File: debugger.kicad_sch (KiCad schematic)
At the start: 29 parts, among them J5 SM03B-SRSS-TB, J7 Conn_ARM_JTAG_SWD_10, J8 Conn_ST_STDC14, J9 SM03B-SRSS-TB

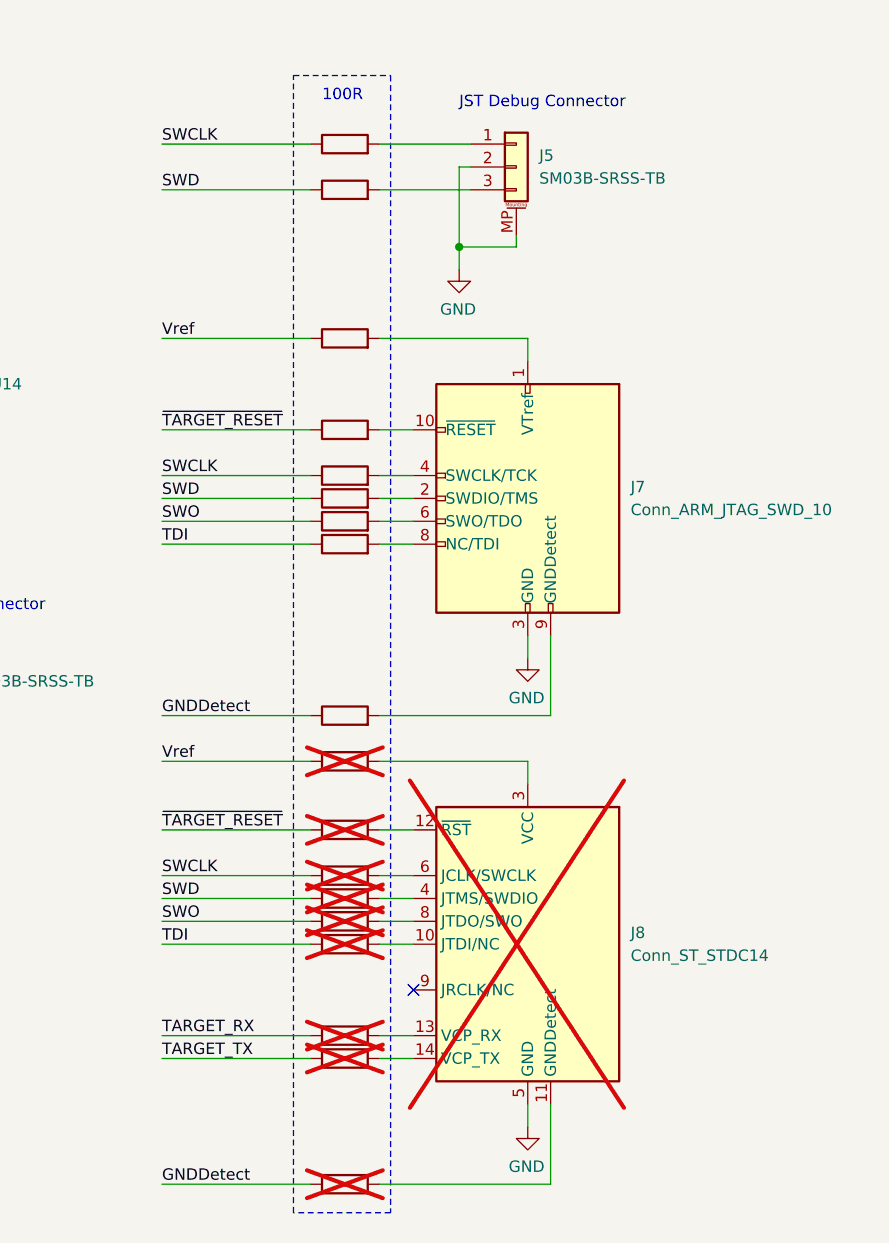
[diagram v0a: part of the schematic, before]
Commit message: Layout Tester and USB Hub
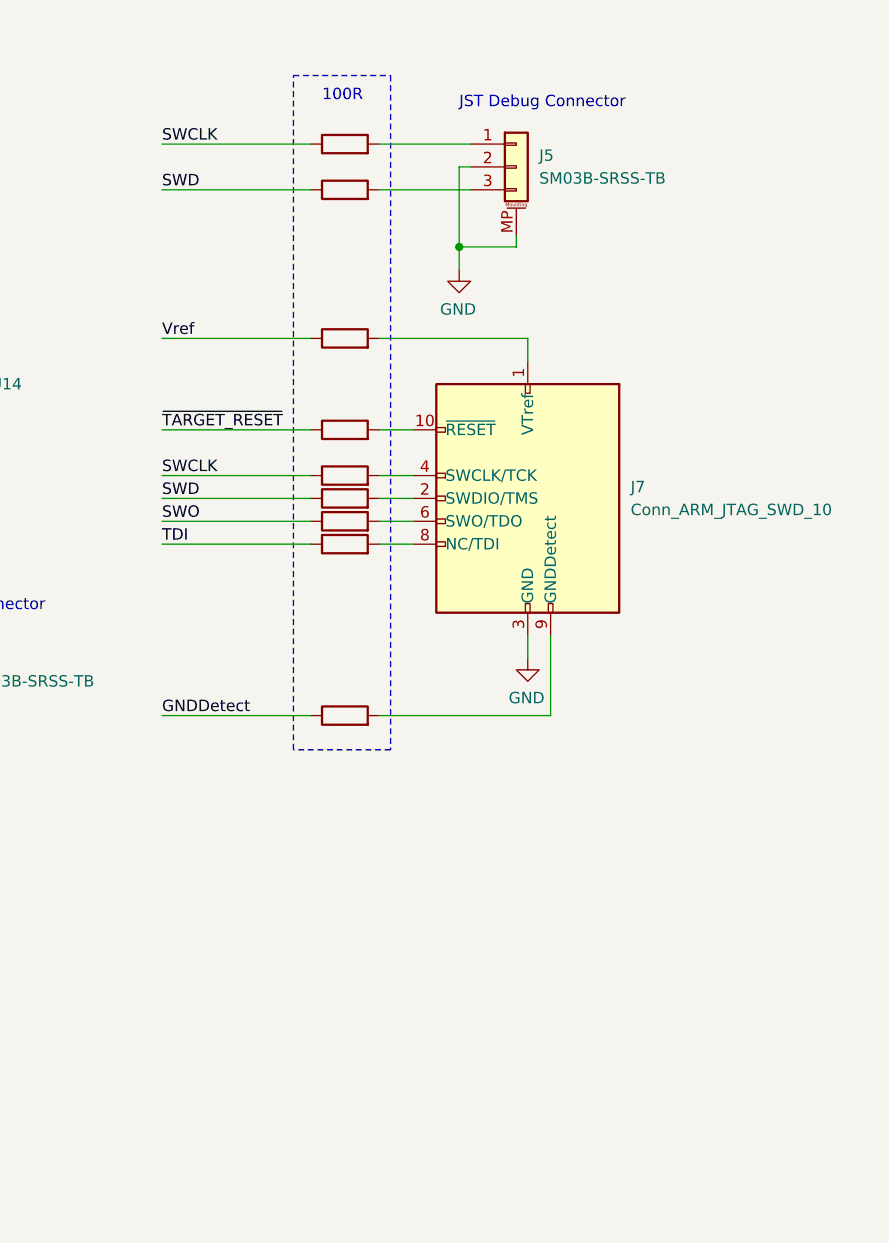
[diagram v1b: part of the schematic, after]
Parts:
- removed J8: Conn_ST_STDC14, Connector_PinHeader_1.27mm:PinHeader_2x07_P1.27mm_Vertical_SMD, symbol Connector:Conn_ST_STDC14
- removed R75, R76, R77, R78, R79, R80, R82, R83, R84: 100R, Resistor_SMD:R_0402_1005Metric_Pad0.72x0.64mm_HandSolder, symbol Device:R
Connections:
- no-connect marks 34 -> 33
